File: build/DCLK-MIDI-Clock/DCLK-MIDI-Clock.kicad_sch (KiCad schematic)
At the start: 32 parts, among them J1 MIDI OUT, J2 Jack-DC, J3 MIDI OUT, J5 Conn_02x04_Odd_Even, J6 Conn_02x04_Odd_Even, SW4 RotaryEncoder_Switch_MP, U2 CAP1206-x-SL

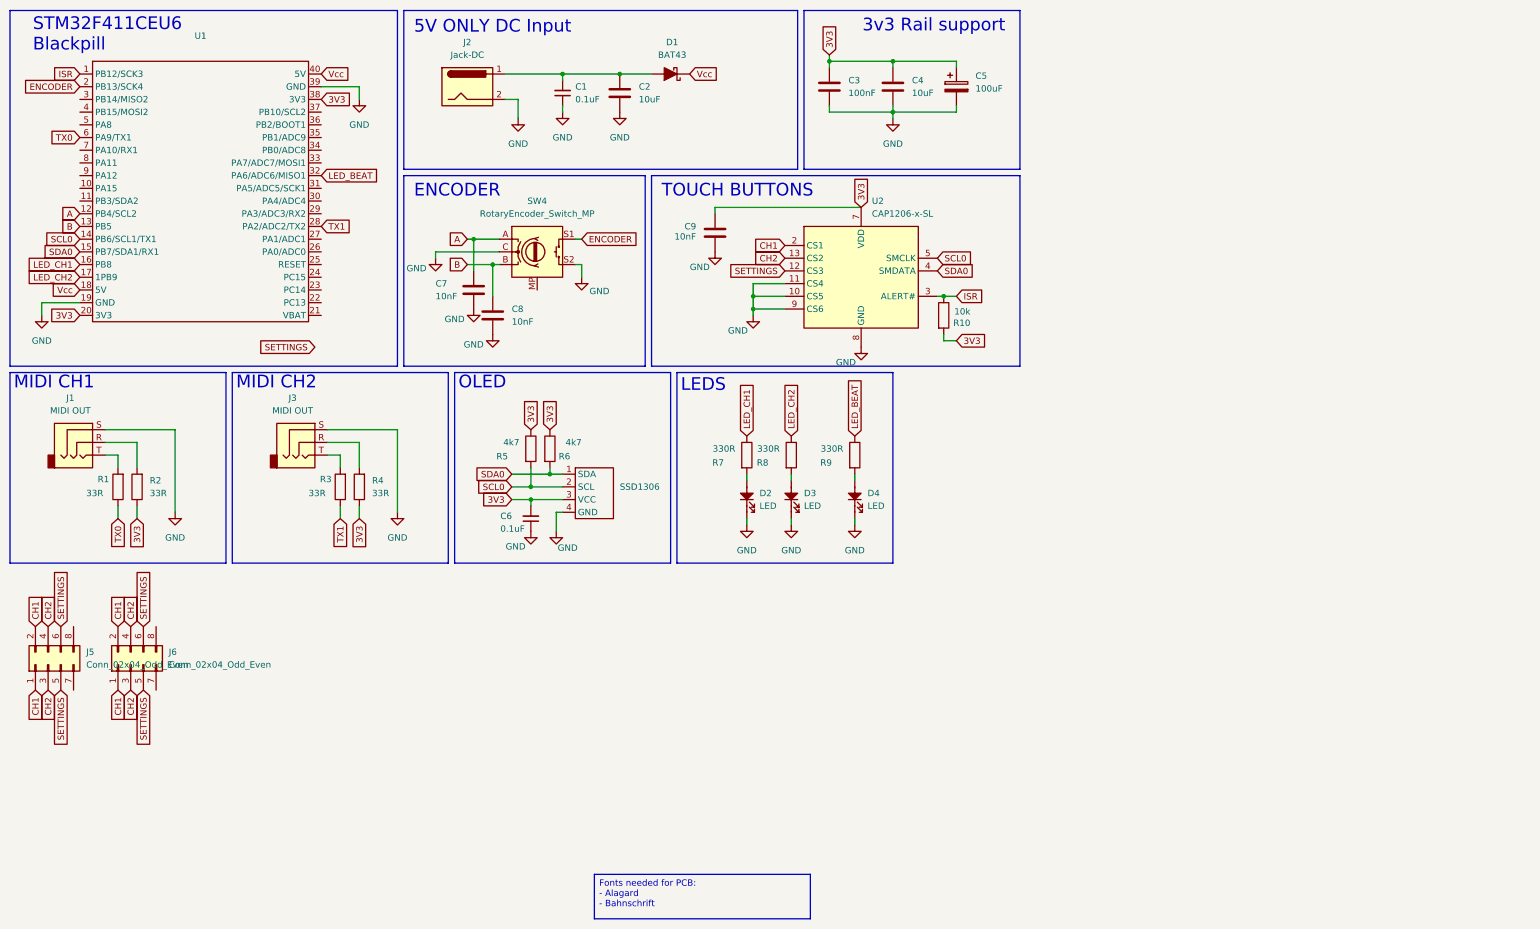
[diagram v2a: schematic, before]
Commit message: SYNC OUT
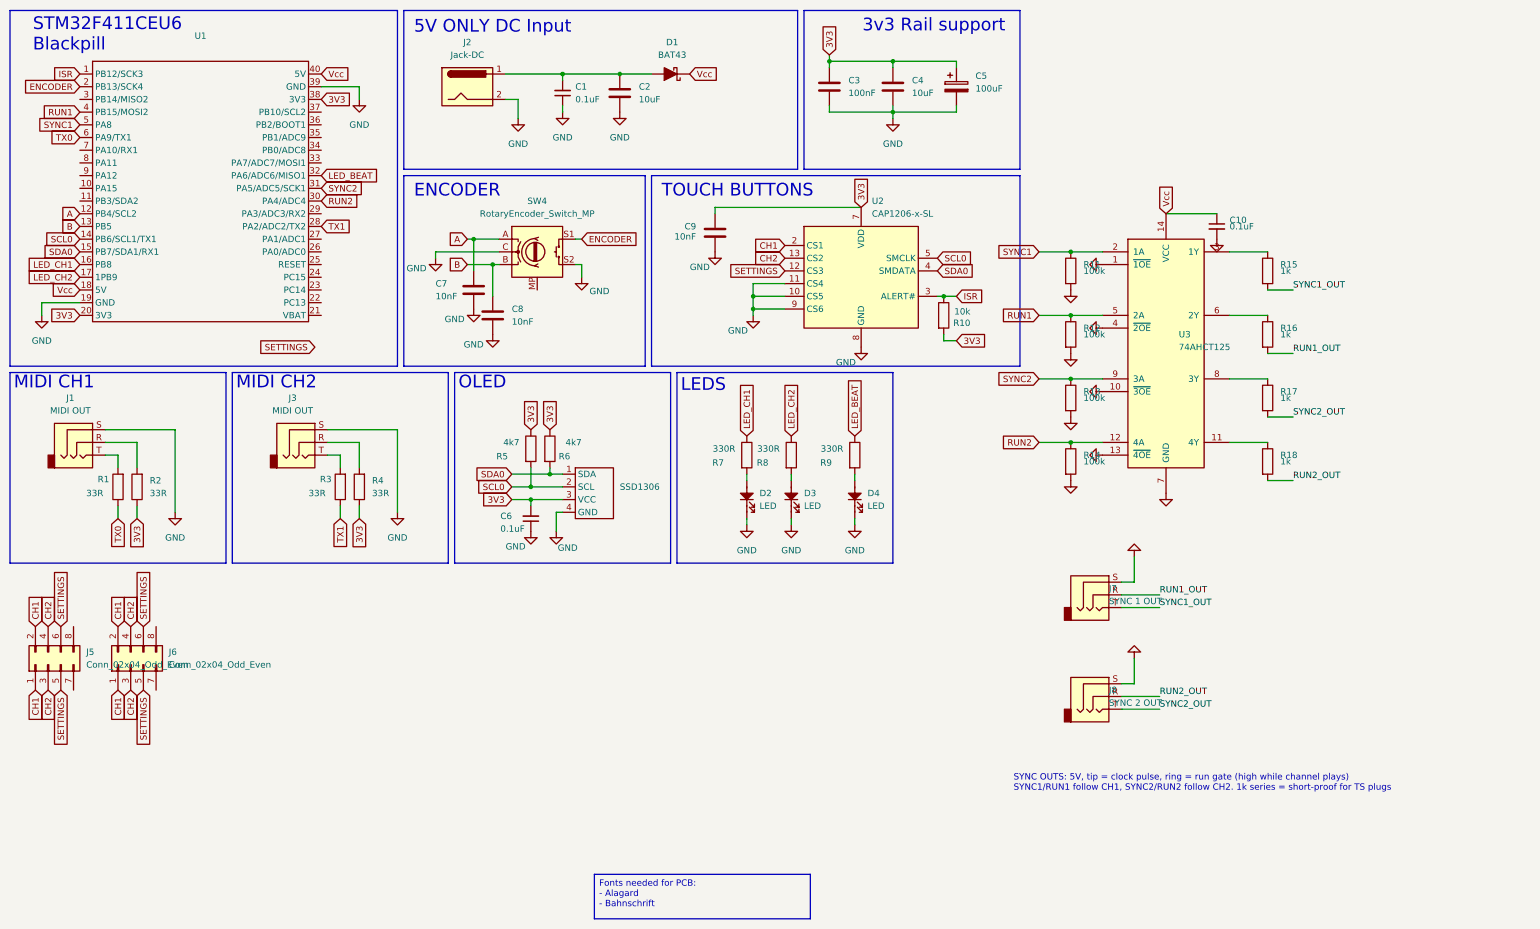
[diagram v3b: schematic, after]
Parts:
- added C10: 100nF, Capacitor_SMD:C_0603_1608Metric, symbol PCM_4ms_Capacitor:100nF_0603_16V
- added J7: SYNC 1 OUT, audioConnectors_Edit:Jack_3.5mm_CUI_SJ1-3525N_Horizontal_edit, symbol Connector_Audio:AudioJack3
- added J8: SYNC 2 OUT, audioConnectors_Edit:Jack_3.5mm_CUI_SJ1-3525N_Horizontal_edit, symbol Connector_Audio:AudioJack3
- added R11, R12, R13, R14: 100k, Resistor_SMD:R_0402_1005Metric, symbol PCM_4ms_Resistor:10k_0402
- added R15, R16, R17, R18: 1k, Resistor_SMD:R_0402_1005Metric, symbol PCM_4ms_Resistor:10k_0402
- added U3: 74AHCT125, Package_SO:SOIC-14_3.9x8.7mm_P1.27mm, symbol DCLK:74AHCT125
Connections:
- net GND: now also C10.2, J7.S, J8.S, R11.2, R12.2, R13.2, R14.2, U3.1 (~{1OE}), U3.10 (~{3OE}), U3.13 (~{4OE}), U3.4 (~{2OE}), U3.7 (GND)
- net Vcc: now also C10.1, U3.14 (VCC)
- net RUN2: now reaches U1.30 (PA4/ADC4)
- net RUN2: now also R14.1, U3.12 (4A)
- net SYNC2: now reaches U1.31 (PA5/ADC5/SCK1)
- net SYNC2: now also R13.1, U3.9 (3A)
- net RUN1: now reaches U1.4 (PB15/MOSI2)
- net RUN1: now also R12.1, U3.5 (2A)
- net SYNC1: now reaches U1.5 (PA8)
- net SYNC1: now also R11.1, U3.2 (1A)
- new net: R18.1, U3.11 (4Y)
- new net: R15.1, U3.3 (1Y)
- new net: R16.1, U3.6 (2Y)
- new net: R17.1, U3.8 (3Y)
- new net RUN1_OUT: J7.R, R16.2
- new net RUN2_OUT: J8.R, R18.2
- new net SYNC1_OUT: J7.T, R15.2
- new net SYNC2_OUT: J8.T, R17.2
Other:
- note added: "SYNC OUTS: 5V, tip = clock pulse, ring = run gate (high while channel plays) SYNC1/RUN1 follow CH1, SYNC2/RUN2 follow CH2. 1k series = short-proof for TS plugs"
